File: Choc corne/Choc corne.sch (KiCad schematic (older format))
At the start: 46 parts, among them J1 MJ-4PP-9, SW1 SW_PUSH, U1 Elite-C

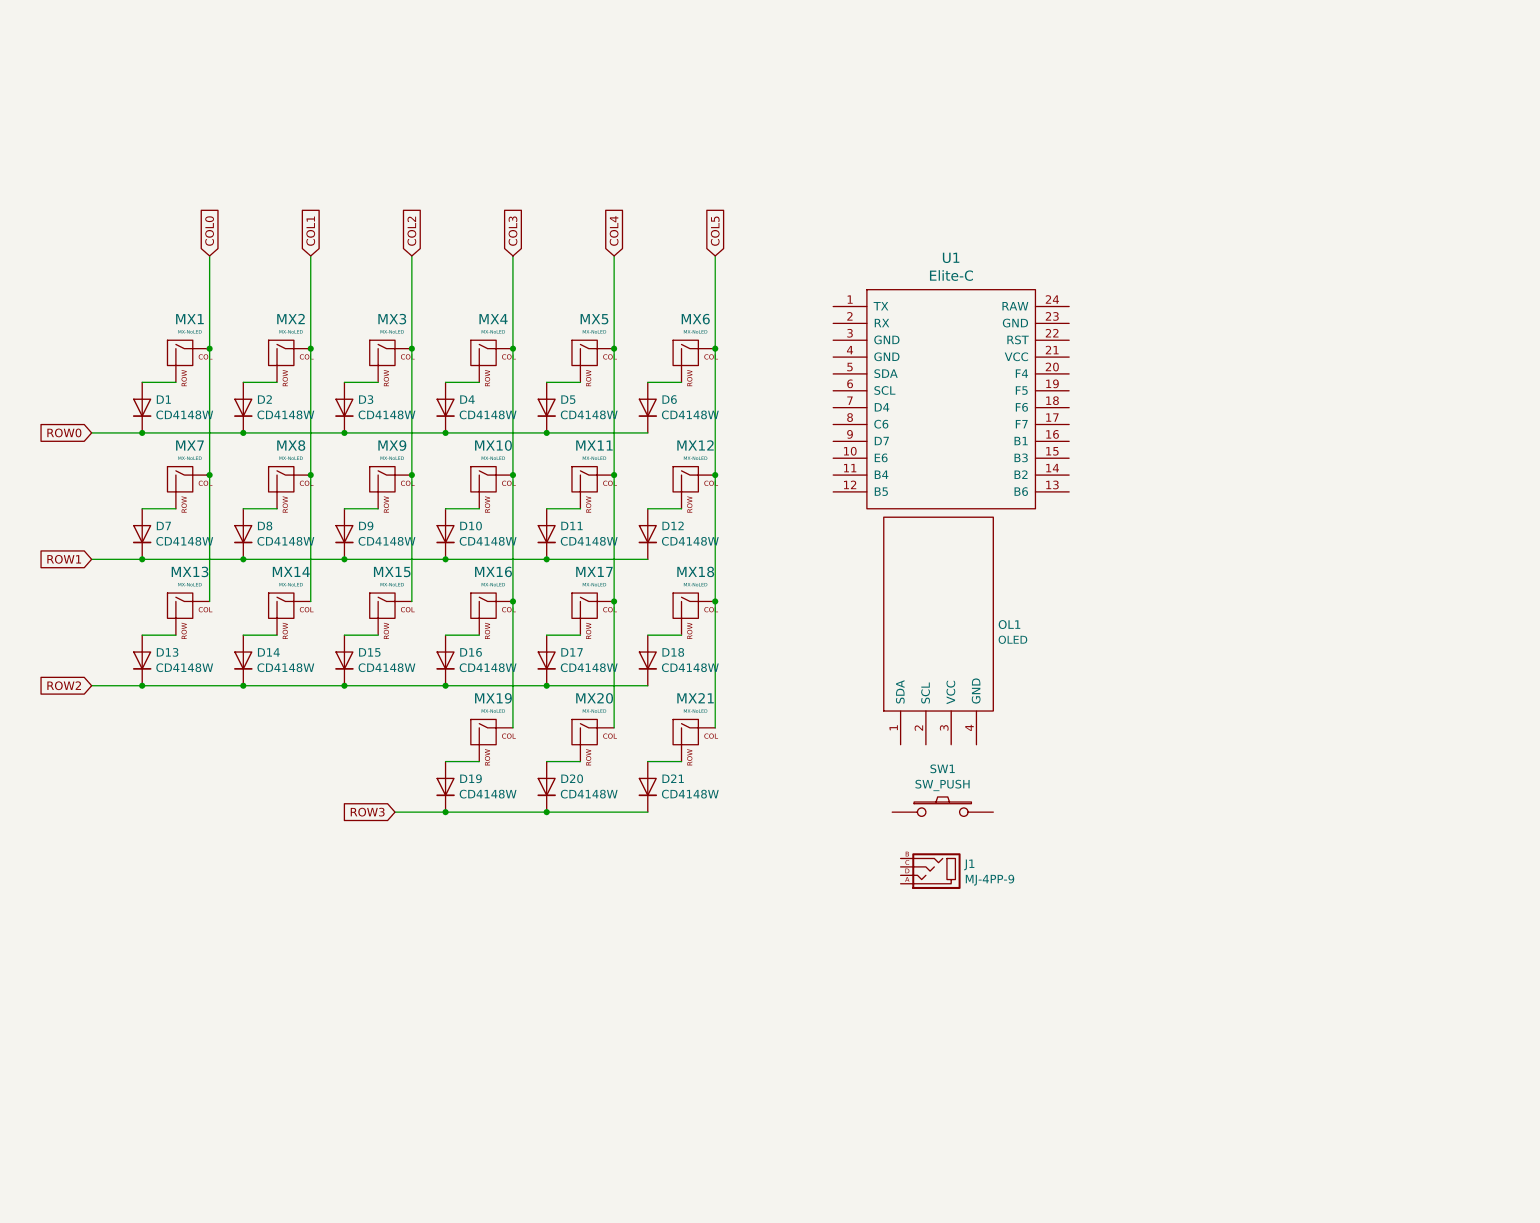
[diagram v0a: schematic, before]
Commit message: big update
whatever
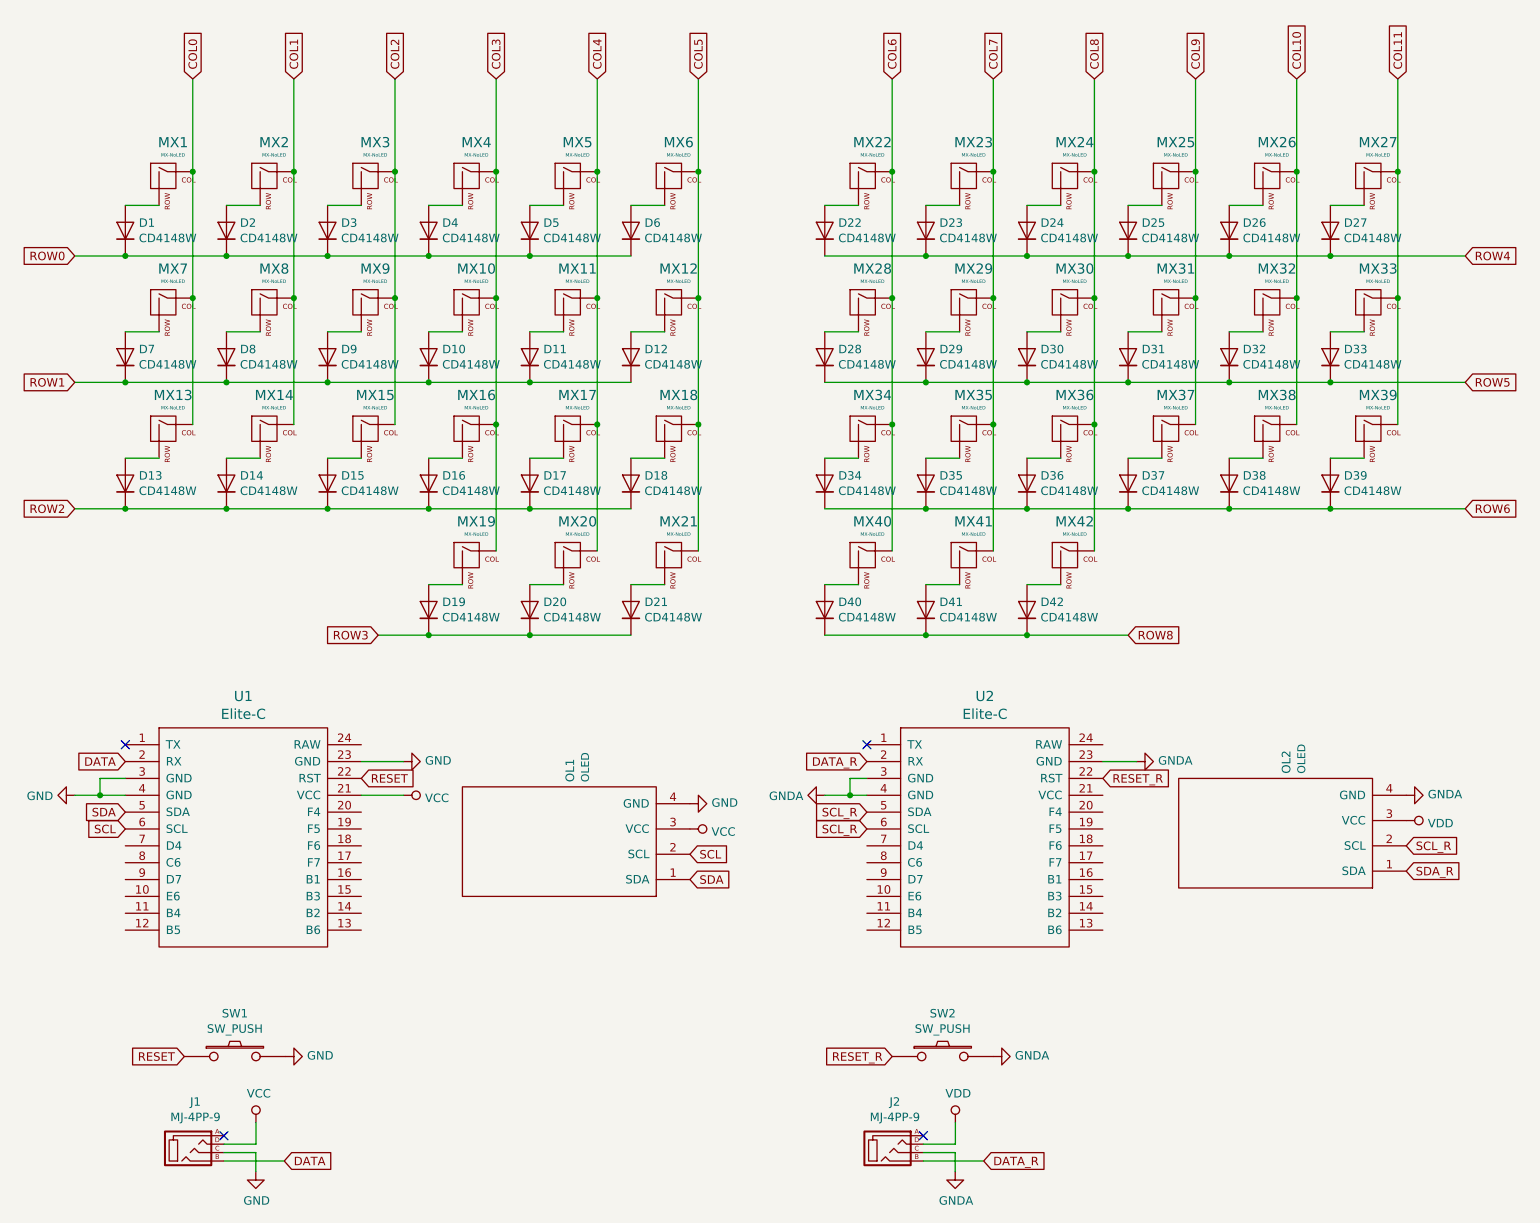
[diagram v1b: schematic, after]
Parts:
- added D22, D23, D24, D25, D26, D27, D28, D29, D30, D31, D32, D33, D34, D35, D36, D37, D38, D39, D40, D41, D42: CD4148W, Diode_SMD:D_0805_2012Metric, symbol Diode:CD4148W
- added J2: MJ-4PP-9, Keebio-Parts:TRRS-PJ-320A, symbol kbd:MJ-4PP-9
- added MX22, MX23, MX24, MX25, MX26, MX27, MX28, MX29, MX30, MX31, MX32, MX33, MX34, MX35, MX36, MX37, MX38, MX39, MX41, MX42: MX-NoLED, kbd:CherryMX_ChocV2_1u, symbol MX_Alps_Hybrid:MX-NoLED
- added MX40: MX-NoLED, kbd:CherryMX_ChocV2_1.5u, symbol MX_Alps_Hybrid:MX-NoLED
- added OL2: OLED, kbd:OLED_1side, symbol kbd:OLED
- added SW2: SW_PUSH, kbd:ResetSW_1side, symbol kbd:SW_PUSH
- added U2: Elite-C, Keebio-Parts:Elite-C, symbol promicro:ProMicro
- J1: footprint (none) -> Keebio-Parts:TRRS-PJ-320A
- MX1, MX10, MX11, MX12, MX13, MX14, MX15, MX16, MX17, MX18, MX19, MX2, MX20, MX3, MX4, MX5, MX6, MX7, MX8, MX9: footprint Keebio-Parts:Kailh-PG1350-1u-NoLED -> kbd:CherryMX_ChocV2_1u
- MX21: footprint Keebio-Parts:Kailh-PG1350-1.5u -> kbd:CherryMX_ChocV2_1.5u
- OL1: footprint (none) -> kbd:OLED_1side
- SW1: footprint (none) -> kbd:ResetSW_1side
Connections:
- net DATA: now reaches U1.2 (RX)
- net DATA: now also J1.B
- net VCC: now reaches U1.21 (VCC)
- net VCC: now also J1.D, OL1.3 (VCC)
- net RESET: now reaches U1.22 (RST)
- net RESET: now also SW1.1
- net GND: now reaches U1.23 (GND)
- net GND: now also J1.C, OL1.4 (GND), SW1.2, U1.3 (GND), U1.4 (GND)
- net SDA: now reaches U1.5 (SDA)
- net SDA: now also OL1.1 (SDA)
- net SCL: now reaches U1.6 (SCL)
- net SCL: now also OL1.2 (SCL)
- new net: D22.2 (A), MX22.2 (ROW)
- new net: D23.2 (A), MX23.2 (ROW)
- new net: D24.2 (A), MX24.2 (ROW)
- new net: D25.2 (A), MX25.2 (ROW)
- new net: D26.2 (A), MX26.2 (ROW)
- new net: D27.2 (A), MX27.2 (ROW)
- new net: D28.2 (A), MX28.2 (ROW)
- new net: D29.2 (A), MX29.2 (ROW)
- new net: D30.2 (A), MX30.2 (ROW)
- new net: D31.2 (A), MX31.2 (ROW)
- new net: D32.2 (A), MX32.2 (ROW)
- new net: D33.2 (A), MX33.2 (ROW)
- new net: D34.2 (A), MX34.2 (ROW)
- new net: D35.2 (A), MX35.2 (ROW)
- new net: D36.2 (A), MX36.2 (ROW)
- new net: D37.2 (A), MX37.2 (ROW)
- new net: D38.2 (A), MX38.2 (ROW)
- new net: D39.2 (A), MX39.2 (ROW)
- new net: D40.2 (A), MX40.2 (ROW)
- new net: D41.2 (A), MX41.2 (ROW)
- new net: D42.2 (A), MX42.2 (ROW)
- new net COL10: MX26.1 (COL), MX32.1 (COL), MX38.1 (COL)
- new net COL11: MX27.1 (COL), MX33.1 (COL), MX39.1 (COL)
- new net COL6: MX22.1 (COL), MX28.1 (COL), MX34.1 (COL), MX40.1 (COL)
- new net COL7: MX23.1 (COL), MX29.1 (COL), MX35.1 (COL), MX41.1 (COL)
- new net COL8: MX24.1 (COL), MX30.1 (COL), MX36.1 (COL), MX42.1 (COL)
- new net COL9: MX25.1 (COL), MX31.1 (COL), MX37.1 (COL)
- new net DATA_R: J2.B, U2.2 (RX)
- new net GNDA: J2.C, OL2.4 (GND), SW2.2, U2.23 (GND), U2.3 (GND), U2.4 (GND)
- new net RESET_R: SW2.1, U2.22 (RST)
- new net ROW4: D22.1 (K), D23.1 (K), D24.1 (K), D25.1 (K), D26.1 (K), D27.1 (K)
- new net ROW5: D28.1 (K), D29.1 (K), D30.1 (K), D31.1 (K), D32.1 (K), D33.1 (K)
- new net ROW6: D34.1 (K), D35.1 (K), D36.1 (K), D37.1 (K), D38.1 (K), D39.1 (K)
- new net ROW8: D40.1 (K), D41.1 (K), D42.1 (K)
- new net SCL_R: OL2.2 (SCL), U2.5 (SDA), U2.6 (SCL)
- new net SDA_R: OL2.1 (SDA)
- new net VDD: J2.D, OL2.3 (VCC)
- no-connect marks 0 -> 4
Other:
- moved on the sheet: D1, D10, D11, D12, D13, D14, D15, D16, D17, D18, D19, D2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
